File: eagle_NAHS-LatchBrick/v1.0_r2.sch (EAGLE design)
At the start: 39 parts, among them IC1 ESP12F, IC2 ATTINY212-SSNR, IC3 TP4056, IC4 DW01A, IC5 FT232RL, J1 10118194-0001LF, Q1 8205A

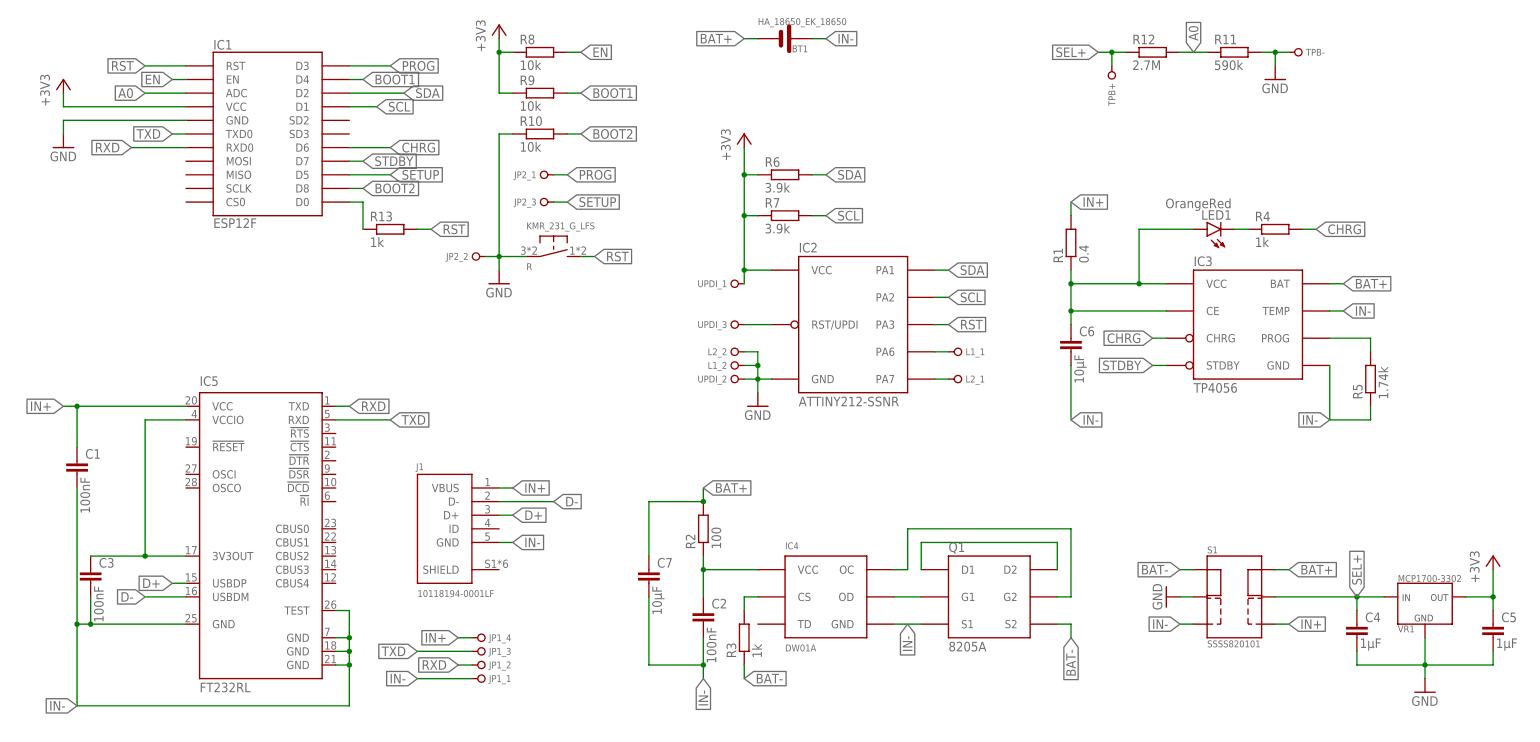
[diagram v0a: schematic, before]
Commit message: saving
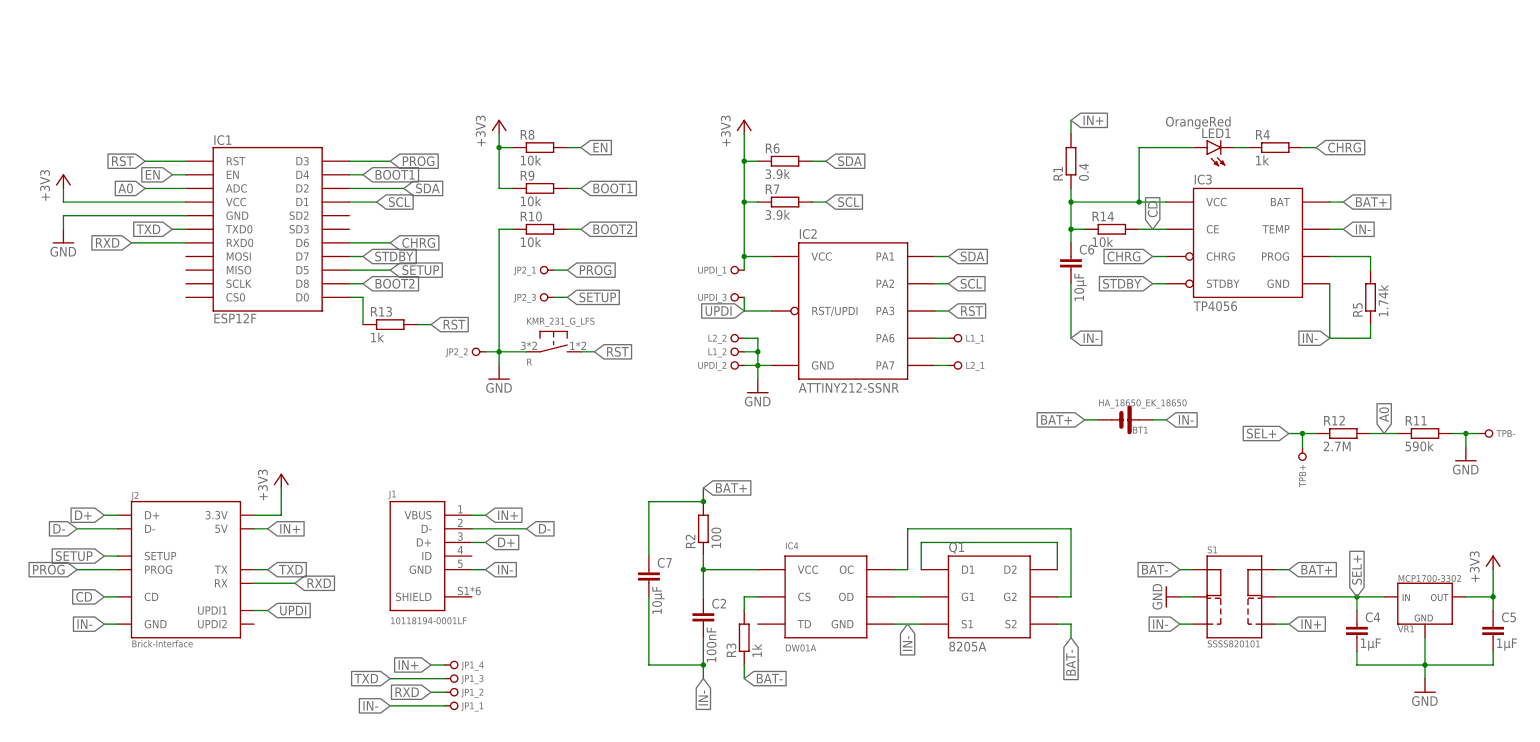
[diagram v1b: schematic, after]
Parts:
- removed C1, C3: 100nF, rcl:C-EUC0805
- removed IC5: FT232RL, ftdichip:FT232RL
- added J2: Brick-Interface, no_molex:NAHS-BRICK-INTERFACE_B-SIDE
- added R14: 10k, rcl:R-EU_R0805
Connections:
- removed net VCCIO: C3.1, IC5.3V3OUT, IC5.VCCIO
- new net CD: IC3.CE, J2.CD, R14.2
- net +3V3: now also J2.3.3V
- net D+: now also J2.D+; no longer IC5.USBDP
- net D-: now also J2.D-; no longer IC5.USBDM
- net IN+: now also J2.5V; no longer C1.1, IC5.VCC
- net IN-: now also J2.GND; no longer C1.2, C3.2, IC5.GND, IC5.GND@1, IC5.GND@2, IC5.GND@A, IC5.TEST
- net N$1: now also R14.1; no longer IC3.CE
- net PROG: now also J2.PROG
- net RXD: now also J2.RX; no longer IC5.TXD
- net SETUP: now also J2.SETUP
- net TXD: now also J2.TX; no longer IC5.RXD
- net UPDI: now also J2.UPDI1
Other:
- moved on the sheet: BT1, C6, IC1, IC2, IC3, J1, JP1_1, JP1_2, JP1_3, JP1_4, JP2_1, JP2_2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
